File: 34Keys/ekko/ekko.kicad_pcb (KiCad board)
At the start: 2 copper layers, 109.8 x 91.3 mm, 25 parts, among them SW10 SW_PUSH, SW11 SW_PUSH, SW12 SW_PUSH, SW14 SW_PUSH, SW15 SW_PUSH, SW16 SW_PUSH, SW17 SW_PUSH, SW18 SW_PUSH, SW2 SW_PUSH, SW20 SW_PUSH, SW21 SW_PUSH, SW3 SW_PUSH, SW4 SW_PUSH, SW5 SW_PUSH, SW6 SW_PUSH, SW8 SW_PUSH, SW9 SW_PUSH, U1 ProMicro

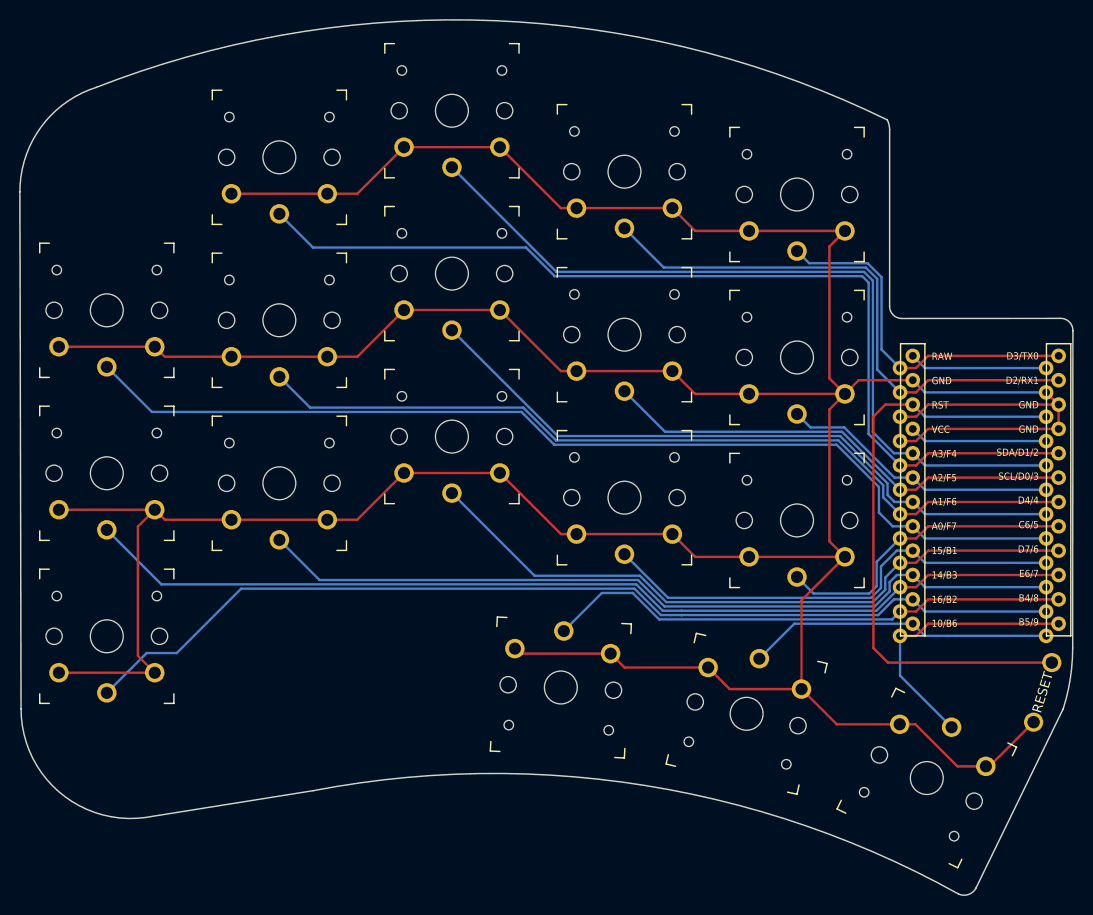
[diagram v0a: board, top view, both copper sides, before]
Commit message: redo some tracks
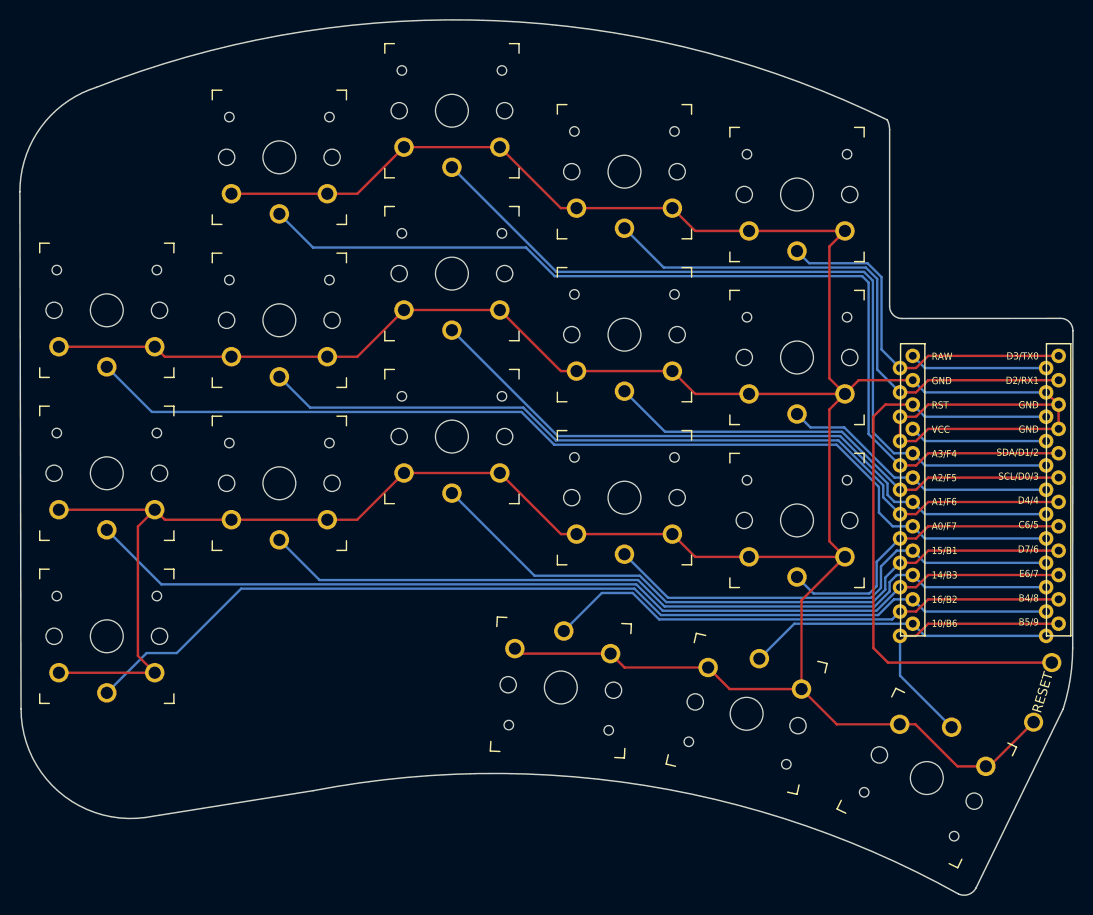
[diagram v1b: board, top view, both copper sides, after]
